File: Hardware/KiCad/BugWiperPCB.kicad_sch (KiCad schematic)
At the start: 0 parts

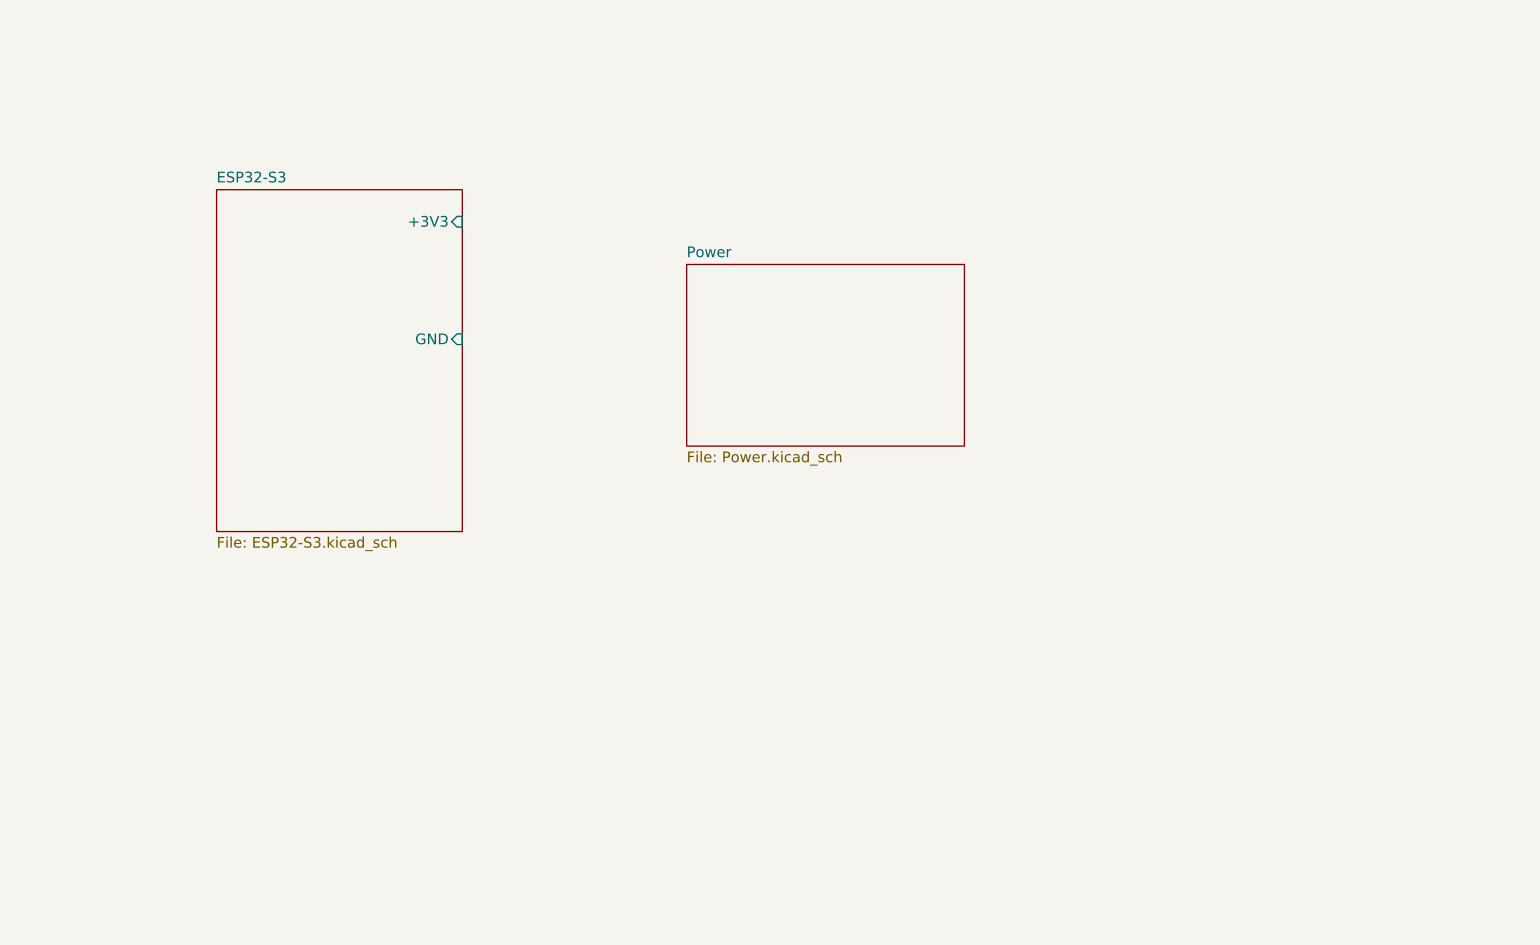
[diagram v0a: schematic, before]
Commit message: update KiCAD files
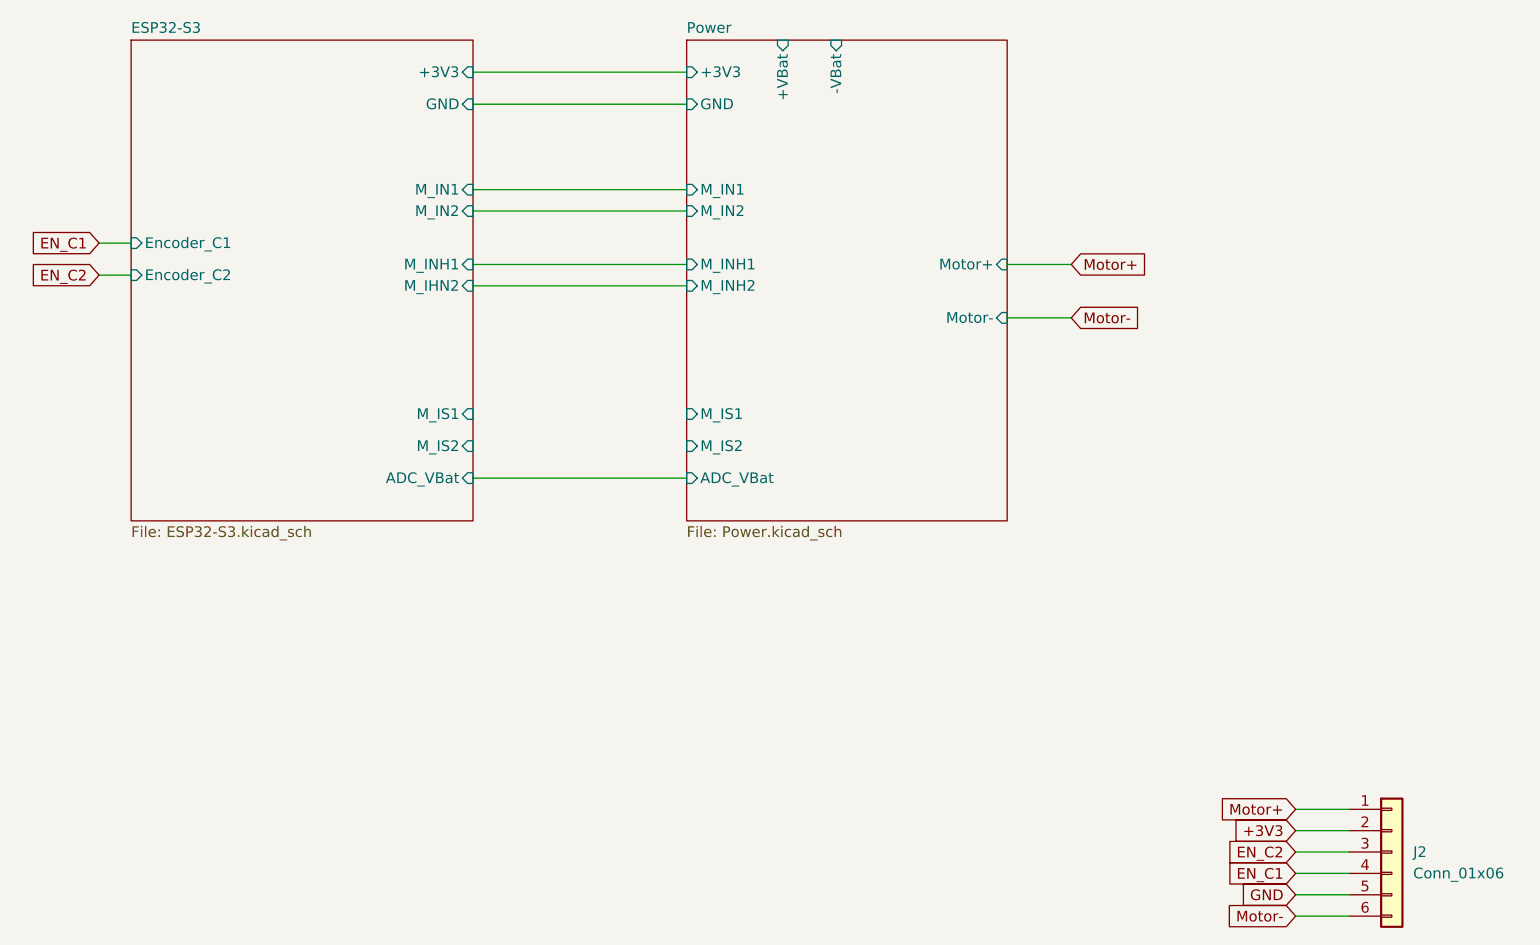
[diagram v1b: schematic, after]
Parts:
- added J2: Conn_01x06, symbol Connector_Generic:Conn_01x06
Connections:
- new net +3V3: J2.2 (Pin_2)
- new net EN_C1: J2.4 (Pin_4)
- new net EN_C2: J2.3 (Pin_3)
- new net GND: J2.5 (Pin_5)
- new net Motor+: J2.1 (Pin_1)
- new net Motor-: J2.6 (Pin_6)
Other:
- sheet ESP32-S3 ports: added ADC_VBat, Encoder_C1, Encoder_C2, M_IHN2, M_IN1, M_IN2, M_INH1, M_IS1, M_IS2; removed none
- sheet Power ports: added +3V3, +VBat, -VBat, ADC_VBat, GND, M_IN1, M_IN2, M_INH1, M_INH2, M_IS1, M_IS2, Motor+, Motor-; removed none
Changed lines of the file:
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@@
 (kicad_sch (version 20230121) (generator eeschema)
   (paper "A4")
-  (sheet (at 142.24 73.66) (size 33.02 21.59) (fields_autoplaced)
+  (wire (pts (xy 214.63 140.97) (xy 220.98 140.97))
+    (stroke (width 0) (type default))
+  )
+  (wire (pts (xy 180.34 73.66) (xy 187.96 73.66))
+    (stroke (width 0) (type default))
+  )
+  (wire (pts (xy 116.84 76.2) (xy 142.24 76.2))
+    (stroke (width 0) (type default))
+  )
+  (wire (pts (xy 214.63 138.43) (xy 220.98 138.43))
+    (stroke (width 0) (type default))
+  )
+  (wire (pts (xy 116.84 64.77) (xy 142.24 64.77))
+    (stroke (width 0) (type default))
+  )
+  (wire (pts (xy 214.63 143.51) (xy 220.98 143.51))
+    (stroke (width 0) (type default))
+  )
+  (wire (pts (xy 180.34 80.01) (xy 187.96 80.01))
+    (stroke (width 0) (type default))
+  )
+  (wire (pts (xy 214.63 151.13) (xy 220.98 151.13))
+    (stroke (width 0) (type default))
+  )
+  (wire (pts (xy 116.84 54.61) (xy 142.24 54.61))
+    (stroke (width 0) (type default))
+  )
+  (wire (pts (xy 72.39 74.93) (xy 76.2 74.93))
+    (stroke (width 0) (type default))
+  )
+  (wire (pts (xy 214.63 148.59) (xy 220.98 148.59))
+    (stroke (width 0) (type default))
+  )
+  (wire (pts (xy 116.84 99.06) (xy 142.24 99.06))
+    (stroke (width 0) (type default))
+  )
+  (wire (pts (xy 116.84 73.66) (xy 142.24 73.66))
+    (stroke (width 0) (type default))
+  )
+  (wire (pts (xy 116.84 50.8) (xy 142.24 50.8))
+    (stroke (width 0) (type default))
+  )
+  (wire (pts (xy 72.39 71.12) (xy 76.2 71.12))
+    (stroke (width 0) (type default))
+  )
+  (wire (pts (xy 214.63 146.05) (xy 220.98 146.05))
+    (stroke (width 0) (type default))
+  )
+  (wire (pts (xy 116.84 67.31) (xy 142.24 67.31))
+    (stroke (width 0) (type default))
+  )
+  (global_label "EN_C1" (shape input) (at 214.63 146.05 180) (fields_autoplaced)
+    (effects (font (size 1.27 1.27)) (justify right))
+    (property "Intersheetrefs" "${INTERSHEET_REFS}" (at 205.7182 146.05 0)
+      (effects (font (size 1.27 1.27)) (justify right) hide)
+    )
+  )
+  (global_label "Motor-" (shape input) (at 214.63 151.13 180) (fields_autoplaced)
+    (effects (font (size 1.27 1.27)) (justify right))
+    (property "Intersheetrefs" "${INTERSHEET_REFS}" (at 204.8111 151.13 0)
+      (effects (font (size 1.27 1.27)) (justify right) hide)
+    )
+  )
+  (global_label "+3V3" (shape input) (at 214.63 140.97 180) (fields_autoplaced)
+    (effects (font (size 1.27 1.27)) (justify right))
+    (property "Intersheetrefs" "${INTERSHEET_REFS}" (at 206.5648 140.97 0)
+      (effects (font (size 1.27 1.27)) (justify right) hide)
+    )
+  )
+  (global_label "Motor+" (shape input) (at 214.63 138.43 180) (fields_autoplaced)
+    (effects (font (size 1.27 1.27)) (justify right))
+    (property "Intersheetrefs" "${INTERSHEET_REFS}" (at 204.8111 138.43 0)
+      (effects (font (size 1.27 1.27)) (justify right) hide)
+    )
+  )
+  (global_label "GND" (shape input) (at 214.63 148.59 180) (fields_autoplaced)
+    (effects (font (size 1.27 1.27)) (justify right))
+    (property "Intersheetrefs" "${INTERSHEET_REFS}" (at 207.7743 148.59 0)
+      (effects (font (size 1.27 1.27)) (justify right) hide)
+    )
+  )
+  (global_label "Motor+" (shape input) (at 187.96 73.66 0) (fields_autoplaced)
+    (effects (font (size 1.27 1.27)) (justify left))
+    (property "Intersheetrefs" "${INTERSHEET_REFS}" (at 197.7789 73.66 0)
+      (effects (font (size 1.27 1.27)) (justify left) hide)
+    )
+  )
+  (global_label "Motor-" (shape input) (at 187.96 80.01 0) (fields_autoplaced)
+    (effects (font (size 1.27 1.27)) (justify left))
+    (property "Intersheetrefs" "${INTERSHEET_REFS}" (at 197.7789 80.01 0)
+      (effects (font (size 1.27 1.27)) (justify left) hide)
+    )
+  )
+  (global_label "EN_C2" (shape input) (at 72.39 74.93 180) (fields_autoplaced)
+    (effects (font (size 1.27 1.27)) (justify right))
+    (property "Intersheetrefs" "${INTERSHEET_REFS}" (at 63.4782 74.93 0)
+      (effects (font (size 1.27 1.27)) (justify right) hide)
+    )
+  )
+  (global_label "EN_C2" (shape input) (at 214.63 143.51 180) (fields_autoplaced)
+    (effects (font (size 1.27 1.27)) (justify right))
+    (property "Intersheetrefs" "${INTERSHEET_REFS}" (at 205.7182 143.51 0)
+      (effects (font (size 1.27 1.27)) (justify right) hide)
+    )
+  )
+  (global_label "EN_C1" (shape input) (at 72.39 71.12 180) (fields_autoplaced)
+    (effects (font (size 1.27 1.27)) (justify right))
+    (property "Intersheetrefs" "${INTERSHEET_REFS}" (at 63.4782 71.12 0)
+      (effects (font (size 1.27 1.27)) (justify right) hide)
+    )
+  )
+  (symbol (lib_id "Connector_Generic:Conn_01x06") (at 226.06 143.51 0) (unit 1)
+    (in_bom yes) (on_board yes) (dnp no) (fields_autoplaced)
+    (property "Reference" "J2" (at 228.6 143.51 0)
+      (effects (font (size 1.27 1.27)) (justify left))
+    )
+    (property "Value" "Conn_01x06" (at 228.6 146.05 0)
+      (effects (font (size 1.27 1.27)) (justify left))
+    )
+    (property "Footprint" "" (at 226.06 143.51 0)
+      (effects (font (size 1.27 1.27)) hide)
+    )
+    (property "Datasheet" "~" (at 226.06 143.51 0)
+      (effects (font (size 1.27 1.27)) hide)
+    )
+    (pin "2")
+    (pin "1")
+    (pin "6")
+    (pin "4")
+    (pin "5")
+    (pin "3")
+    (instances
+      (project "BugWiperPCB"
+        (path "/d31a15bd-db02-4d4c-9593-17c596d3182c"
+          (reference "J2") (unit 1)
+        )
+      )
+    )
+  )
+  (sheet (at 142.24 46.99) (size 38.1 57.15) (fields_autoplaced)
     (stroke (width 0.1524) (type solid))
     (fill (color 0 0 0 0.0000))
-    (property "Sheetname" "Power" (at 142.24 72.9484 0)
+    (property "Sheetname" "Power" (at 142.24 46.2784 0)
       (effects (font (size 1.27 1.27)) (justify left bottom))
     )
-    (property "Sheetfile" "Power.kicad_sch" (at 142.24 95.8346 0)
+    (property "Sheetfile" "Power.kicad_sch" (at 142.24 104.7246 0)
       (effects (font (size 1.27 1.27)) (justify left top))
+    )
+    (pin "+VBat" input (at 153.67 46.99 90)
+      (effects (font (size 1.27 1.27)) (justify right))
+    )
+    (pin "Motor+" input (at 180.34 73.66 0)
+      (effects (font (size 1.27 1.27)) (justify right))
+    )
+    (pin "Motor-" input (at 180.34 80.01 0)
+      (effects (font (size 1.27 1.27)) (justify right))
+    )
+    (pin "ADC_VBat" input (at 142.24 99.06 180)
+      (effects (font (size 1.27 1.27)) (justify left))
+    )
+    (pin "-VBat" input (at 160.02 46.99 90)
+      (effects (font (size 1.27 1.27)) (justify right))
+    )
+    (pin "M_IN1" input (at 142.24 64.77 180)
+      (effects (font (size 1.27 1.27)) (justify left))
+    )
+    (pin "M_IS2" input (at 142.24 95.25 180)
+      (effects (font (size 1.27 1.27)) (justify left))
+    )
+    (pin "M_IS1" input (at 142.24 91.44 180)
+      (effects (font (size 1.27 1.27)) (justify left))
+    )
+    (pin "M_IN2" input (at 142.24 67.31 180)
+      (effects (font (size 1.27 1.27)) (justify left))
+    )
+    (pin "M_INH2" input (at 142.24 76.2 180)
+      (effects (font (size 1.27 1.27)) (justify left))
+    )
+    (pin "M_INH1" input (at 142.24 73.66 180)
+      (effects (font (size 1.27 1.27)) (justify left))
+    )
+    (pin "+3V3" input (at 142.24 50.8 180)
+      (effects (font (size 1.27 1.27)) (justify left))
+    )
+    (pin "GND" input (at 142.24 54.61 180)
+      (effects (font (size 1.27 1.27)) (justify left))
     )
     (instances
@@
     )
   )
-  (sheet (at 86.36 64.77) (size 29.21 40.64) (fields_autoplaced)
+  (sheet (at 76.2 46.99) (size 40.64 57.15) (fields_autoplaced)
     (stroke (width 0.1524) (type solid))
-    (fill (color 0 0 0 0.0000))
-    (property "Sheetname" "ESP32-S3" (at 86.36 64.0584 0)
+    (fill (color 0 194 0 0.5400))
+    (property "Sheetname" "ESP32-S3" (at 76.2 46.2784 0)
       (effects (font (size 1.27 1.27)) (justify left bottom))
     )
-    (property "Sheetfile" "ESP32-S3.kicad_sch" (at 86.36 105.9946 0)
+    (property "Sheetfile" "ESP32-S3.kicad_sch" (at 76.2 104.7246 0)
       (effects (font (size 1.27 1.27)) (justify left top))
     )
-    (pin "+3V3" input (at 115.57 68.58 0)
-      (effects (font (size 1.27 1.27)) (justify right))
-    )
-    (pin "GND" input (at 115.57 82.55 0)
-      (effects (font (size 1.27 1.27)) (justify right))
-    )
+    (pin "+3V3" input (at 116.84 50.8 0)
+      (effects (font (size 1.27 1.27)) (justify right))
+    )
+    (pin "GND" input (at 116.84 54.61 0)
+      (effects (font (size 1.27 1.27)) (justify right))
+    )
+    (pin "Encoder_C1" input (at 76.2 71.12 180)
+      (effects (font (size 1.27 1.27)) (justify left))
+    )
+    (pin "Encoder_C2" input (at 76.2 74.93 180)
+      (effects (font (size 1.27 1.27)) (justify left))
+    )
+    (pin "ADC_VBat" input (at 116.84 99.06 0)
+      (effects (font (size 1.27 1.27)) (justify right))
+    )
+    (pin "M_IS2" input (at 116.84 95.25 0)
+      (effects (font (size 1.27 1.27)) (justify right))
+    )
+    (pin "M_IS1" input (at 116.84 91.44 0)
+      (effects (font (size 1.27 1.27)) (justify right))
+    )
+    (pin "M_IN1" input (at 116.84 64.77 0)
+      (effects (font (size 1.27 1.27)) (justify right))
+    )
+    (pin "M_IN2" input (at 116.84 67.31 0)
+      (effects (font (size 1.27 1.27)) (justify right))
+    )
+    (pin "M_INH1" input (at 116.84 73.66 0)
+      (effects (font (size 1.27 1.27)) (justify right))
+    )
+    (pin "M_IHN2" input (at 116.84 76.2 0)
+      (effects (font (size 1.27 1.27)) (justify right))
+    )
